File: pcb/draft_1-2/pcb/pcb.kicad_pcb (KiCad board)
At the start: 2 copper layers, 29.5 x 39.4 mm, 35 parts, among them J1 USB4110-GF-A, J2 SWD, U1 H3LIS200DLTR, U2 ATSAML21J16B-AUT, U3 BQ25155

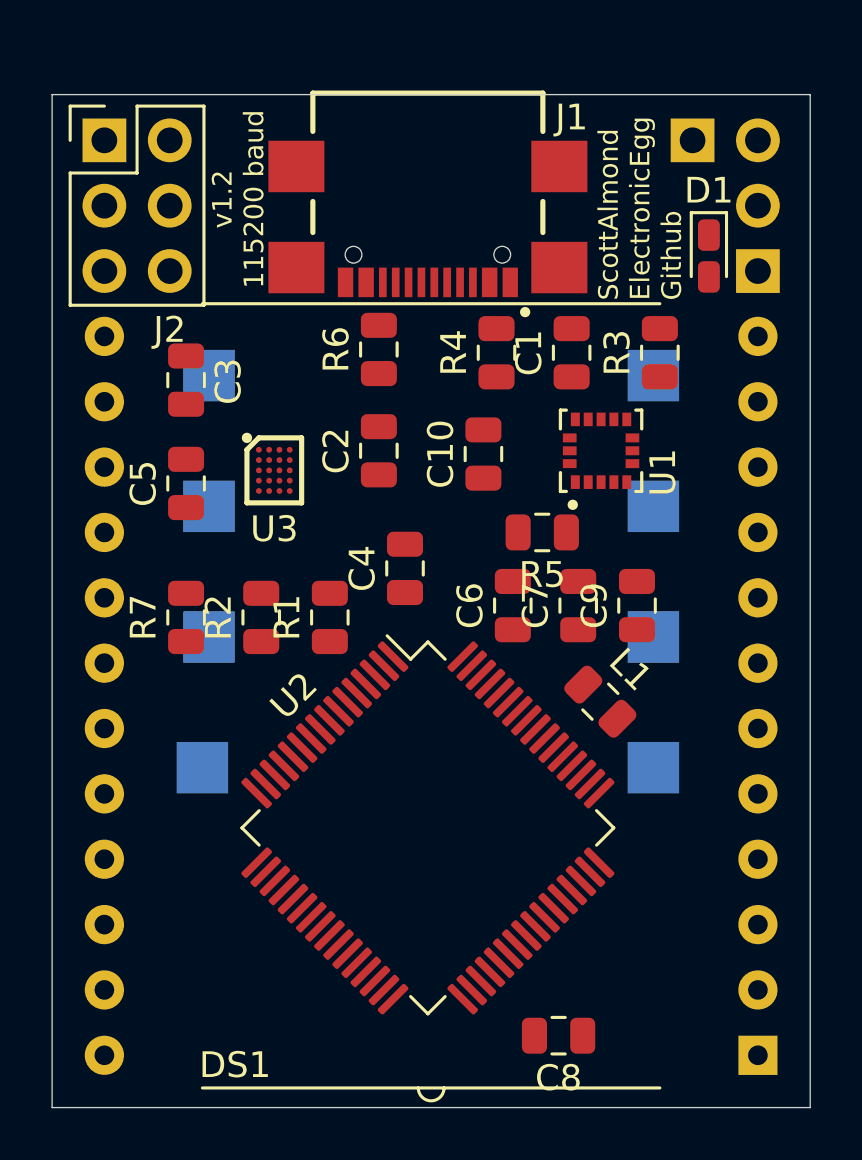
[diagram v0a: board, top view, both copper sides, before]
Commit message: v1.2 draft
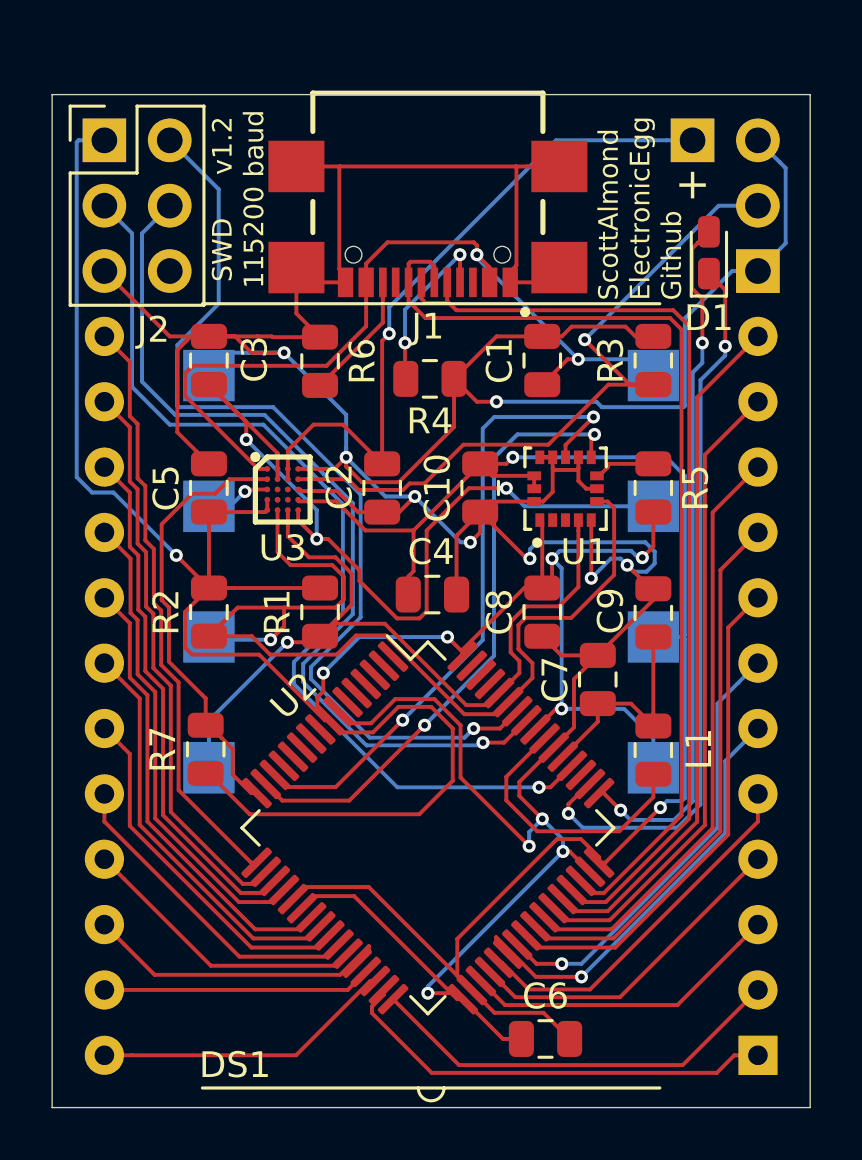
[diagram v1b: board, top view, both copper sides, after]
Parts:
- moved C6 16.9 mm to (146.2, 124.3), turned to 180 degrees
- moved C8 16.5 mm to (146.1, 107.7), turned to 270 degrees
- moved R7 5.18 mm to (133.0, 113.1), turned to 270 degrees
- moved R5 4.65 mm to (150.4, 102.9), turned to 270 degrees
- moved C7 2.97 mm to (148.2, 110.4)
- moved L1 2.79 mm to (150.4, 113.1), turned to 270 degrees
- moved R4 2.78 mm to (141.7, 98.7), turned to 180 degrees
- moved R6 2.33 mm to (137.4, 98.0), turned to 270 degrees
- moved R2 2.04 mm to (133.1, 107.7)
- moved U1 2.02 mm to (147.0, 102.9)
- moved C4 1.47 mm to (141.8, 107.1), turned to 0 degrees
- moved C2 1.45 mm to (139.8, 102.9), turned to 270 degrees
- moved C10 1.32 mm to (143.6, 102.9)
- moved C1 1.18 mm to (146.1, 98.0)
- moved C3 1.17 mm to (133.1, 98.0)
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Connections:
- U2 pad 14: INT3 -> INT1
- U2 pad 16: INT1 -> INT3
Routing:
- net GND: track 0.00 -> 184.9 mm, vias 0 -> 12
- net VREF: track 0.00 -> 94.1 mm, vias 0 -> 6
- net +3V3: track 0.00 -> 63.7 mm, vias 0 -> 2
- net SDA: track 0.00 -> 41.3 mm, vias 0 -> 1
- net D+: track 0.00 -> 38.5 mm
- net ~RESET: track 0.00 -> 38.2 mm, vias 0 -> 1
- net SWDIO: track 0.00 -> 37.7 mm, vias 0 -> 1
- net D-: track 0.00 -> 37.5 mm
- net SWCLK: track 0.00 -> 35.3 mm, vias 0 -> 1
- net +5V: track 0.00 -> 32.9 mm, vias 0 -> 2
- net Net-(C3-Pad2): track 0.00 -> 32.8 mm, vias 0 -> 3
- net SCL: track 0.00 -> 32.2 mm, vias 0 -> 1
- net Net-(D1-Pad1): track 0.00 -> 28.6 mm, vias 0 -> 2
- net Net-(R3-Pad1): track 0.00 -> 28.0 mm, vias 0 -> 1
- net Net-(D1-Pad2): track 0.00 -> 27.1 mm, vias 0 -> 2
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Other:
- board text added: "SWD v1.2 115200 baud"
- board text removed: "v1.2 115200 baud"
